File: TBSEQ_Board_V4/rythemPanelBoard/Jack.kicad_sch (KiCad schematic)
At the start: 1 part, among them J1 Conn_01x05

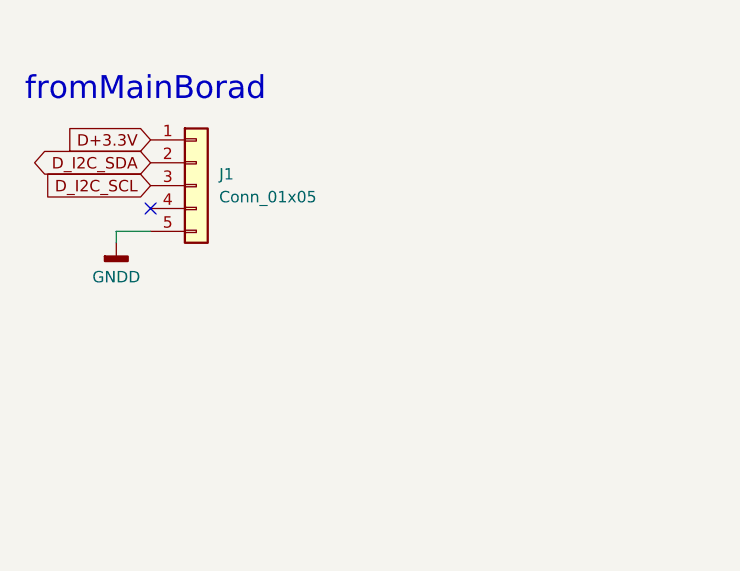
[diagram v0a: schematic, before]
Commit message: TBSEQ_BoardV4
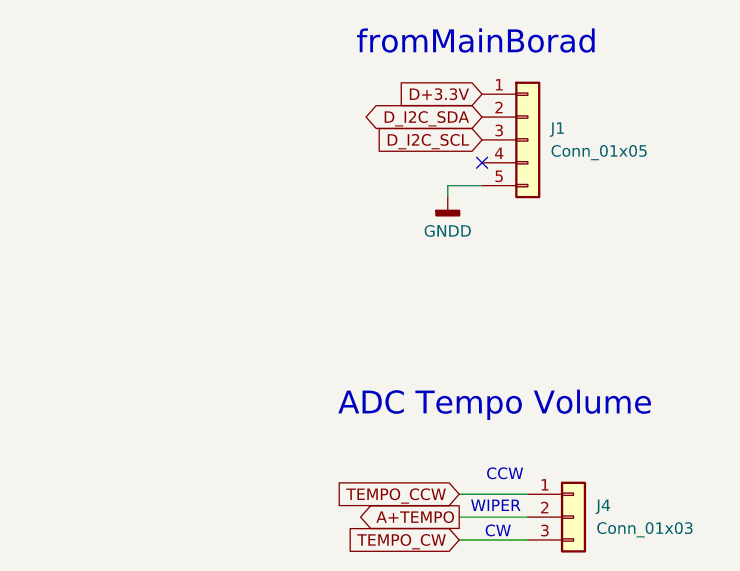
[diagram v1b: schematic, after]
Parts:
- added J4: Conn_01x03, Connector_PinSocket_2.54mm:PinSocket_1x03_P2.54mm_Vertical, symbol Connector_Generic:Conn_01x03
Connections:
- new net A+TEMPO: J4.2 (Pin_2)
- new net TEMPO_CCW: J4.1 (Pin_1)
- new net TEMPO_CW: J4.3 (Pin_3)
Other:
- note added: "ADC Tempo Volume"
- note added: "CCW"
- note added: "CW"
- note added: "WIPER"
- moved on the sheet: J1
